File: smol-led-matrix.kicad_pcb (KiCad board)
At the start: 4 copper layers, 61.8 x 88.2 mm, 381 parts, among them J1 USB_C_Receptacle_USB2.0, J2 TagConnect_TC2030_SWD, Q1 FS8205, Q2 AO3401A, SW1 SW_Push, SW2 SW_Push, U1 STM32L433CBTx, U2 TP4054, U3 DW01+G, U4 XC6206P332MR

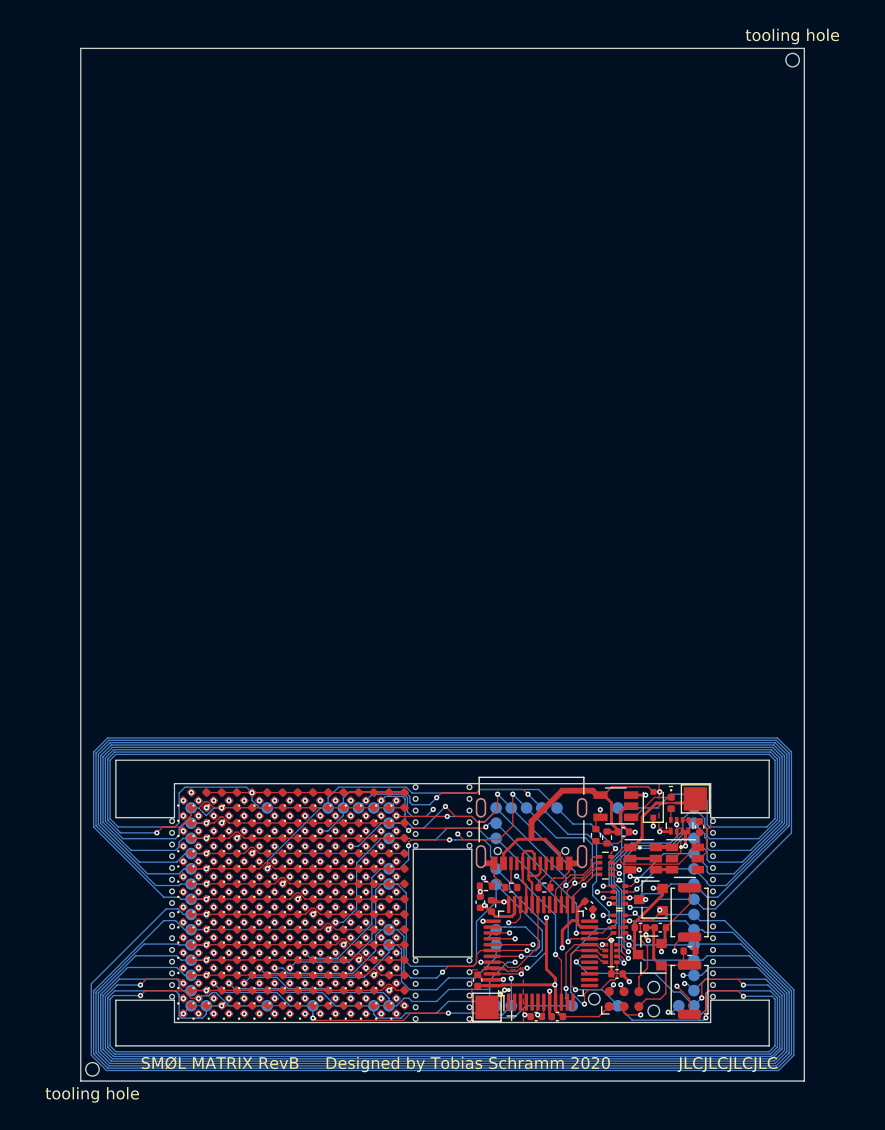
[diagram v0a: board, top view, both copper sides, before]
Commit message: Repanelize
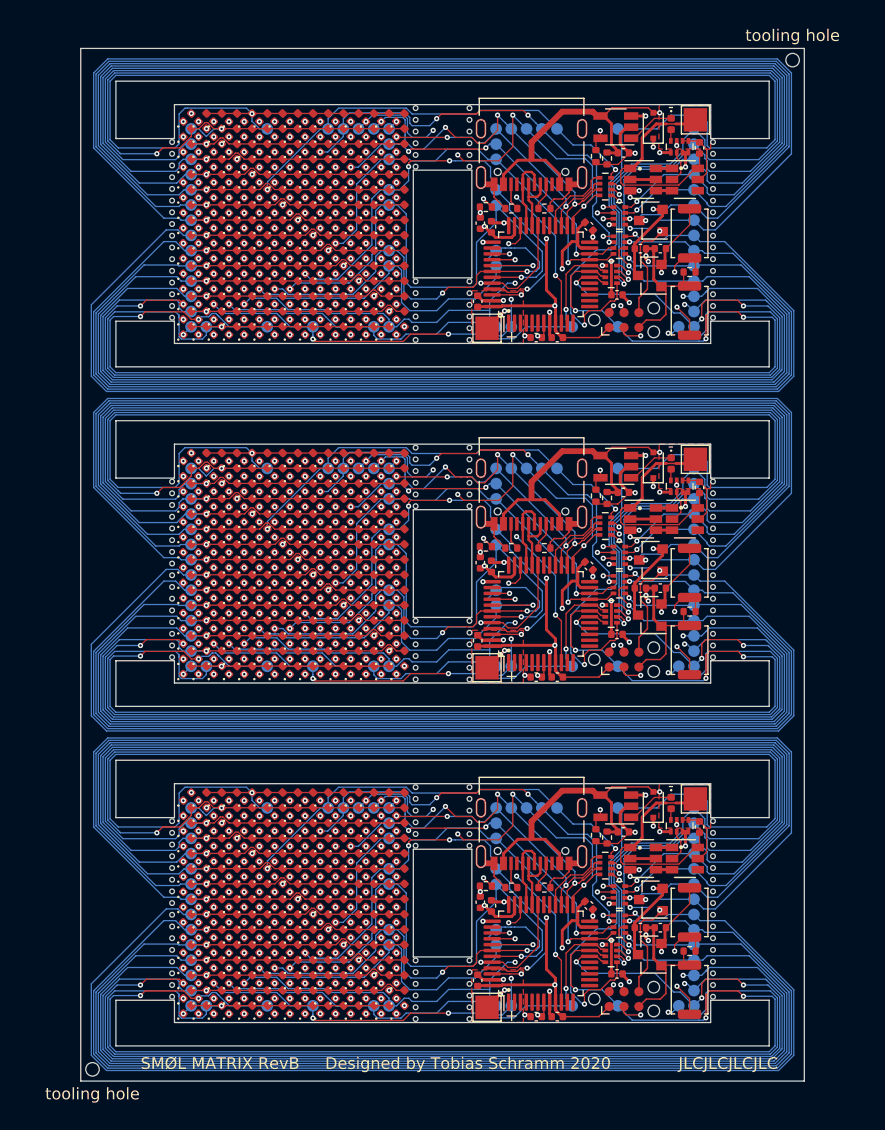
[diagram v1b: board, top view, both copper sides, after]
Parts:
- added C1: 100nF, Capacitor_SMD:C_0402_1005Metric, F.Cu at (94.8, 86.5)
- added C1: 100nF, Capacitor_SMD:C_0402_1005Metric, F.Cu at (94.8, 115.5)
- added C10: 10uF, Capacitor_SMD:C_0402_1005Metric, F.Cu at (99.9, 82.8)
- added C10: 10uF, Capacitor_SMD:C_0402_1005Metric, F.Cu at (99.9, 111.8)
- added C11: 100nF, Capacitor_SMD:C_0402_1005Metric, F.Cu at (88.2, 76.7)
- added C11: 100nF, Capacitor_SMD:C_0402_1005Metric, F.Cu at (88.2, 105.7)
- added C2: 100nF, Capacitor_SMD:C_0402_1005Metric, F.Cu at (88.0, 83.4)
- added C2: 100nF, Capacitor_SMD:C_0402_1005Metric, F.Cu at (88.0, 112.4)
- added C3: 1uF, Capacitor_SMD:C_0402_1005Metric, F.Cu at (100.5, 70.7)
- added C3: 1uF, Capacitor_SMD:C_0402_1005Metric, F.Cu at (100.5, 99.7)
- added C4: 100nF, Capacitor_SMD:C_0402_1005Metric, F.Cu at (107.0, 70.3)
- added C4: 100nF, Capacitor_SMD:C_0402_1005Metric, F.Cu at (107.0, 99.3)
- added C5: 100nF, Capacitor_SMD:C_0402_1005Metric, F.Cu at (93.0, 86.5)
- added C5: 100nF, Capacitor_SMD:C_0402_1005Metric, F.Cu at (93.0, 115.5)
- added C6: 1uF, Capacitor_SMD:C_0402_1005Metric, F.Cu at (101.9, 78.9)
- added C6: 1uF, Capacitor_SMD:C_0402_1005Metric, F.Cu at (101.9, 107.9)
- added C7: 1uF, Capacitor_SMD:C_0402_1005Metric, F.Cu at (103.6, 78.9)
- added C7: 1uF, Capacitor_SMD:C_0402_1005Metric, F.Cu at (103.6, 107.9)
- added C8: 100nF, Capacitor_SMD:C_0402_1005Metric, F.Cu at (89.2, 77.0)
- added C8: 100nF, Capacitor_SMD:C_0402_1005Metric, F.Cu at (89.2, 106.0)
- added C9: 100nF, Capacitor_SMD:C_0402_1005Metric, F.Cu at (97.5, 77.0)
- added C9: 100nF, Capacitor_SMD:C_0402_1005Metric, F.Cu at (97.5, 106.0)
- added D1: LED, LED_SMD:LED_0402_1005Metric, F.Cu at (63.2, 67.7)
- added D1: LED, LED_SMD:LED_0402_1005Metric, F.Cu at (63.2, 96.7)
- added D10: LED, LED_SMD:LED_0402_1005Metric, F.Cu at (63.2, 79.4)
- added D10: LED, LED_SMD:LED_0402_1005Metric, F.Cu at (63.2, 108.4)
- added D100: LED, LED_SMD:LED_0402_1005Metric, F.Cu at (71.0, 79.4)
- added D100: LED, LED_SMD:LED_0402_1005Metric, F.Cu at (71.0, 108.4)
- added D101: LED, LED_SMD:LED_0402_1005Metric, F.Cu at (71.0, 80.7)
- added D101: LED, LED_SMD:LED_0402_1005Metric, F.Cu at (71.0, 109.7)
- added D102: LED, LED_SMD:LED_0402_1005Metric, F.Cu at (71.0, 82.0)
- added D102: LED, LED_SMD:LED_0402_1005Metric, F.Cu at (71.0, 111.0)
- added D103: LED, LED_SMD:LED_0402_1005Metric, F.Cu at (71.0, 83.3)
- added D103: LED, LED_SMD:LED_0402_1005Metric, F.Cu at (71.0, 112.3)
- added D104: LED, LED_SMD:LED_0402_1005Metric, F.Cu at (71.0, 84.6)
- added D104: LED, LED_SMD:LED_0402_1005Metric, F.Cu at (71.0, 113.6)
- added D105: LED, LED_SMD:LED_0402_1005Metric, F.Cu at (71.0, 85.9)
- added D105: LED, LED_SMD:LED_0402_1005Metric, F.Cu at (71.0, 114.9)
- added D106: LED, LED_SMD:LED_0402_1005Metric, F.Cu at (72.3, 67.7)
- added D106: LED, LED_SMD:LED_0402_1005Metric, F.Cu at (72.3, 96.7)
- added D107: LED, LED_SMD:LED_0402_1005Metric, F.Cu at (72.3, 69.0)
- added D107: LED, LED_SMD:LED_0402_1005Metric, F.Cu at (72.3, 98.0)
- added D108: LED, LED_SMD:LED_0402_1005Metric, F.Cu at (72.3, 70.3)
- added D108: LED, LED_SMD:LED_0402_1005Metric, F.Cu at (72.3, 99.3)
- added D109: LED, LED_SMD:LED_0402_1005Metric, F.Cu at (72.3, 71.6)
- added D109: LED, LED_SMD:LED_0402_1005Metric, F.Cu at (72.3, 100.6)
- added D11: LED, LED_SMD:LED_0402_1005Metric, F.Cu at (63.2, 80.7)
- added D11: LED, LED_SMD:LED_0402_1005Metric, F.Cu at (63.2, 109.7)
- added D110: LED, LED_SMD:LED_0402_1005Metric, F.Cu at (72.3, 72.9)
- added D110: LED, LED_SMD:LED_0402_1005Metric, F.Cu at (72.3, 101.9)
- added D111: LED, LED_SMD:LED_0402_1005Metric, F.Cu at (72.3, 74.2)
- added D111: LED, LED_SMD:LED_0402_1005Metric, F.Cu at (72.3, 103.2)
- added D112: LED, LED_SMD:LED_0402_1005Metric, F.Cu at (72.3, 75.5)
- added D112: LED, LED_SMD:LED_0402_1005Metric, F.Cu at (72.3, 104.5)
- added D113: LED, LED_SMD:LED_0402_1005Metric, F.Cu at (72.3, 76.8)
- added D113: LED, LED_SMD:LED_0402_1005Metric, F.Cu at (72.3, 105.8)
- added D114: LED, LED_SMD:LED_0402_1005Metric, F.Cu at (72.3, 78.1)
- added D114: LED, LED_SMD:LED_0402_1005Metric, F.Cu at (72.3, 107.1)
- added D115: LED, LED_SMD:LED_0402_1005Metric, F.Cu at (72.3, 79.4)
- added D115: LED, LED_SMD:LED_0402_1005Metric, F.Cu at (72.3, 108.4)
- added D116: LED, LED_SMD:LED_0402_1005Metric, F.Cu at (72.3, 80.7)
- added D116: LED, LED_SMD:LED_0402_1005Metric, F.Cu at (72.3, 109.7)
- added D117: LED, LED_SMD:LED_0402_1005Metric, F.Cu at (72.3, 82.0)
- added D117: LED, LED_SMD:LED_0402_1005Metric, F.Cu at (72.3, 111.0)
- added D118: LED, LED_SMD:LED_0402_1005Metric, F.Cu at (72.3, 83.3)
- added D118: LED, LED_SMD:LED_0402_1005Metric, F.Cu at (72.3, 112.3)
- added D119: LED, LED_SMD:LED_0402_1005Metric, F.Cu at (72.3, 84.6)
- added D119: LED, LED_SMD:LED_0402_1005Metric, F.Cu at (72.3, 113.6)
- added D12: LED, LED_SMD:LED_0402_1005Metric, F.Cu at (63.2, 82.0)
- added D12: LED, LED_SMD:LED_0402_1005Metric, F.Cu at (63.2, 111.0)
- added D120: LED, LED_SMD:LED_0402_1005Metric, F.Cu at (72.3, 85.9)
- added D120: LED, LED_SMD:LED_0402_1005Metric, F.Cu at (72.3, 114.9)
- added D121: LED, LED_SMD:LED_0402_1005Metric, F.Cu at (73.6, 67.7)
- added D121: LED, LED_SMD:LED_0402_1005Metric, F.Cu at (73.6, 96.7)
- added D122: LED, LED_SMD:LED_0402_1005Metric, F.Cu at (73.6, 69.0)
- added D122: LED, LED_SMD:LED_0402_1005Metric, F.Cu at (73.6, 98.0)
- added D123: LED, LED_SMD:LED_0402_1005Metric, F.Cu at (73.6, 70.3)
- added D123: LED, LED_SMD:LED_0402_1005Metric, F.Cu at (73.6, 99.3)
- added D124: LED, LED_SMD:LED_0402_1005Metric, F.Cu at (73.6, 71.6)
- added D124: LED, LED_SMD:LED_0402_1005Metric, F.Cu at (73.6, 100.6)
- added D125: LED, LED_SMD:LED_0402_1005Metric, F.Cu at (73.6, 72.9)
- added D125: LED, LED_SMD:LED_0402_1005Metric, F.Cu at (73.6, 101.9)
- added D126: LED, LED_SMD:LED_0402_1005Metric, F.Cu at (73.6, 74.2)
- added D126: LED, LED_SMD:LED_0402_1005Metric, F.Cu at (73.6, 103.2)
- added D127: LED, LED_SMD:LED_0402_1005Metric, F.Cu at (73.6, 75.5)
- added D127: LED, LED_SMD:LED_0402_1005Metric, F.Cu at (73.6, 104.5)
- added D128: LED, LED_SMD:LED_0402_1005Metric, F.Cu at (73.6, 76.8)
- added D128: LED, LED_SMD:LED_0402_1005Metric, F.Cu at (73.6, 105.8)
- added D129: LED, LED_SMD:LED_0402_1005Metric, F.Cu at (73.6, 78.1)
- added D129: LED, LED_SMD:LED_0402_1005Metric, F.Cu at (73.6, 107.1)
- added D13: LED, LED_SMD:LED_0402_1005Metric, F.Cu at (63.2, 83.3)
- added D13: LED, LED_SMD:LED_0402_1005Metric, F.Cu at (63.2, 112.3)
- added D130: LED, LED_SMD:LED_0402_1005Metric, F.Cu at (73.6, 79.4)
- added D130: LED, LED_SMD:LED_0402_1005Metric, F.Cu at (73.6, 108.4)
- added D131: LED, LED_SMD:LED_0402_1005Metric, F.Cu at (73.6, 80.7)
- added D131: LED, LED_SMD:LED_0402_1005Metric, F.Cu at (73.6, 109.7)
- added D132: LED, LED_SMD:LED_0402_1005Metric, F.Cu at (73.6, 82.0)
- added D132: LED, LED_SMD:LED_0402_1005Metric, F.Cu at (73.6, 111.0)
- added D133: LED, LED_SMD:LED_0402_1005Metric, F.Cu at (73.6, 83.3)
- added D133: LED, LED_SMD:LED_0402_1005Metric, F.Cu at (73.6, 112.3)
- added D134: LED, LED_SMD:LED_0402_1005Metric, F.Cu at (73.6, 84.6)
- added D134: LED, LED_SMD:LED_0402_1005Metric, F.Cu at (73.6, 113.6)
- added D135: LED, LED_SMD:LED_0402_1005Metric, F.Cu at (73.6, 85.9)
- added D135: LED, LED_SMD:LED_0402_1005Metric, F.Cu at (73.6, 114.9)
- added D136: LED, LED_SMD:LED_0402_1005Metric, F.Cu at (74.9, 67.7)
- added D136: LED, LED_SMD:LED_0402_1005Metric, F.Cu at (74.9, 96.7)
- added D137: LED, LED_SMD:LED_0402_1005Metric, F.Cu at (74.9, 69.0)
- added D137: LED, LED_SMD:LED_0402_1005Metric, F.Cu at (74.9, 98.0)
- added D138: LED, LED_SMD:LED_0402_1005Metric, F.Cu at (74.9, 70.3)
- added D138: LED, LED_SMD:LED_0402_1005Metric, F.Cu at (74.9, 99.3)
- added D139: LED, LED_SMD:LED_0402_1005Metric, F.Cu at (74.9, 71.6)
- added D139: LED, LED_SMD:LED_0402_1005Metric, F.Cu at (74.9, 100.6)
- added D14: LED, LED_SMD:LED_0402_1005Metric, F.Cu at (63.2, 84.6)
- added D14: LED, LED_SMD:LED_0402_1005Metric, F.Cu at (63.2, 113.6)
- added D140: LED, LED_SMD:LED_0402_1005Metric, F.Cu at (74.9, 72.9)
- added D140: LED, LED_SMD:LED_0402_1005Metric, F.Cu at (74.9, 101.9)
- added D141: LED, LED_SMD:LED_0402_1005Metric, F.Cu at (74.9, 74.2)
- added D141: LED, LED_SMD:LED_0402_1005Metric, F.Cu at (74.9, 103.2)
- added D142: LED, LED_SMD:LED_0402_1005Metric, F.Cu at (74.9, 75.5)
- added D142: LED, LED_SMD:LED_0402_1005Metric, F.Cu at (74.9, 104.5)
- added D143: LED, LED_SMD:LED_0402_1005Metric, F.Cu at (74.9, 76.8)
- added D143: LED, LED_SMD:LED_0402_1005Metric, F.Cu at (74.9, 105.8)
- added D144: LED, LED_SMD:LED_0402_1005Metric, F.Cu at (74.9, 78.1)
- added D144: LED, LED_SMD:LED_0402_1005Metric, F.Cu at (74.9, 107.1)
- added D145: LED, LED_SMD:LED_0402_1005Metric, F.Cu at (74.9, 79.4)
- added D145: LED, LED_SMD:LED_0402_1005Metric, F.Cu at (74.9, 108.4)
- added D146: LED, LED_SMD:LED_0402_1005Metric, F.Cu at (74.9, 80.7)
- added D146: LED, LED_SMD:LED_0402_1005Metric, F.Cu at (74.9, 109.7)
- added D147: LED, LED_SMD:LED_0402_1005Metric, F.Cu at (74.9, 82.0)
- added D147: LED, LED_SMD:LED_0402_1005Metric, F.Cu at (74.9, 111.0)
- added D148: LED, LED_SMD:LED_0402_1005Metric, F.Cu at (74.9, 83.3)
- added D148: LED, LED_SMD:LED_0402_1005Metric, F.Cu at (74.9, 112.3)
- added D149: LED, LED_SMD:LED_0402_1005Metric, F.Cu at (74.9, 84.6)
- added D149: LED, LED_SMD:LED_0402_1005Metric, F.Cu at (74.9, 113.6)
- added D15: LED, LED_SMD:LED_0402_1005Metric, F.Cu at (63.2, 85.9)
- added D15: LED, LED_SMD:LED_0402_1005Metric, F.Cu at (63.2, 114.9)
- added D150: LED, LED_SMD:LED_0402_1005Metric, F.Cu at (74.9, 85.9)
- added D150: LED, LED_SMD:LED_0402_1005Metric, F.Cu at (74.9, 114.9)
- added D151: LED, LED_SMD:LED_0402_1005Metric, F.Cu at (76.2, 67.7)
- added D151: LED, LED_SMD:LED_0402_1005Metric, F.Cu at (76.2, 96.7)
- added D152: LED, LED_SMD:LED_0402_1005Metric, F.Cu at (76.2, 69.0)
- added D152: LED, LED_SMD:LED_0402_1005Metric, F.Cu at (76.2, 98.0)
- added D153: LED, LED_SMD:LED_0402_1005Metric, F.Cu at (76.2, 70.3)
- added D153: LED, LED_SMD:LED_0402_1005Metric, F.Cu at (76.2, 99.3)
- added D154: LED, LED_SMD:LED_0402_1005Metric, F.Cu at (76.2, 71.6)
- added D154: LED, LED_SMD:LED_0402_1005Metric, F.Cu at (76.2, 100.6)
- added D155: LED, LED_SMD:LED_0402_1005Metric, F.Cu at (76.2, 72.9)
- added D155: LED, LED_SMD:LED_0402_1005Metric, F.Cu at (76.2, 101.9)
- added D156: LED, LED_SMD:LED_0402_1005Metric, F.Cu at (76.2, 74.2)
- added D156: LED, LED_SMD:LED_0402_1005Metric, F.Cu at (76.2, 103.2)
- added D157: LED, LED_SMD:LED_0402_1005Metric, F.Cu at (76.2, 75.5)
- added D157: LED, LED_SMD:LED_0402_1005Metric, F.Cu at (76.2, 104.5)
- added D158: LED, LED_SMD:LED_0402_1005Metric, F.Cu at (76.2, 76.8)
- added D158: LED, LED_SMD:LED_0402_1005Metric, F.Cu at (76.2, 105.8)
- added D159: LED, LED_SMD:LED_0402_1005Metric, F.Cu at (76.2, 78.1)
- added D159: LED, LED_SMD:LED_0402_1005Metric, F.Cu at (76.2, 107.1)
- added D16: LED, LED_SMD:LED_0402_1005Metric, F.Cu at (64.5, 67.7)
- added D16: LED, LED_SMD:LED_0402_1005Metric, F.Cu at (64.5, 96.7)
- added D160: LED, LED_SMD:LED_0402_1005Metric, F.Cu at (76.2, 79.4)
- added D160: LED, LED_SMD:LED_0402_1005Metric, F.Cu at (76.2, 108.4)
- added D161: LED, LED_SMD:LED_0402_1005Metric, F.Cu at (76.2, 80.7)
- added D161: LED, LED_SMD:LED_0402_1005Metric, F.Cu at (76.2, 109.7)
- added D162: LED, LED_SMD:LED_0402_1005Metric, F.Cu at (76.2, 82.0)
- added D162: LED, LED_SMD:LED_0402_1005Metric, F.Cu at (76.2, 111.0)
- added D163: LED, LED_SMD:LED_0402_1005Metric, F.Cu at (76.2, 83.3)
- added D163: LED, LED_SMD:LED_0402_1005Metric, F.Cu at (76.2, 112.3)
- added D164: LED, LED_SMD:LED_0402_1005Metric, F.Cu at (76.2, 84.6)
- added D164: LED, LED_SMD:LED_0402_1005Metric, F.Cu at (76.2, 113.6)
- added D165: LED, LED_SMD:LED_0402_1005Metric, F.Cu at (76.2, 85.9)
- added D165: LED, LED_SMD:LED_0402_1005Metric, F.Cu at (76.2, 114.9)
- added D166: LED, LED_SMD:LED_0402_1005Metric, F.Cu at (77.5, 67.7)
- added D166: LED, LED_SMD:LED_0402_1005Metric, F.Cu at (77.5, 96.7)
- added D167: LED, LED_SMD:LED_0402_1005Metric, F.Cu at (77.5, 69.0)
- added D167: LED, LED_SMD:LED_0402_1005Metric, F.Cu at (77.5, 98.0)
- added D168: LED, LED_SMD:LED_0402_1005Metric, F.Cu at (77.5, 70.3)
- added D168: LED, LED_SMD:LED_0402_1005Metric, F.Cu at (77.5, 99.3)
- added D169: LED, LED_SMD:LED_0402_1005Metric, F.Cu at (77.5, 71.6)
- added D169: LED, LED_SMD:LED_0402_1005Metric, F.Cu at (77.5, 100.6)
- added D17: LED, LED_SMD:LED_0402_1005Metric, F.Cu at (64.5, 69.0)
- added D17: LED, LED_SMD:LED_0402_1005Metric, F.Cu at (64.5, 98.0)
- added D170: LED, LED_SMD:LED_0402_1005Metric, F.Cu at (77.5, 72.9)
- added D170: LED, LED_SMD:LED_0402_1005Metric, F.Cu at (77.5, 101.9)
- added D171: LED, LED_SMD:LED_0402_1005Metric, F.Cu at (77.5, 74.2)
- added D171: LED, LED_SMD:LED_0402_1005Metric, F.Cu at (77.5, 103.2)
- added D172: LED, LED_SMD:LED_0402_1005Metric, F.Cu at (77.5, 75.5)
- added D172: LED, LED_SMD:LED_0402_1005Metric, F.Cu at (77.5, 104.5)
- added D173: LED, LED_SMD:LED_0402_1005Metric, F.Cu at (77.5, 76.8)
- added D173: LED, LED_SMD:LED_0402_1005Metric, F.Cu at (77.5, 105.8)
- added D174: LED, LED_SMD:LED_0402_1005Metric, F.Cu at (77.5, 78.1)
- added D174: LED, LED_SMD:LED_0402_1005Metric, F.Cu at (77.5, 107.1)
- added D175: LED, LED_SMD:LED_0402_1005Metric, F.Cu at (77.5, 79.4)
- added D175: LED, LED_SMD:LED_0402_1005Metric, F.Cu at (77.5, 108.4)
- added D176: LED, LED_SMD:LED_0402_1005Metric, F.Cu at (77.5, 80.7)
- added D176: LED, LED_SMD:LED_0402_1005Metric, F.Cu at (77.5, 109.7)
- added D177: LED, LED_SMD:LED_0402_1005Metric, F.Cu at (77.5, 82.0)
- added D177: LED, LED_SMD:LED_0402_1005Metric, F.Cu at (77.5, 111.0)
- added D178: LED, LED_SMD:LED_0402_1005Metric, F.Cu at (77.5, 83.3)
- added D178: LED, LED_SMD:LED_0402_1005Metric, F.Cu at (77.5, 112.3)
- added D179: LED, LED_SMD:LED_0402_1005Metric, F.Cu at (77.5, 84.6)
- added D179: LED, LED_SMD:LED_0402_1005Metric, F.Cu at (77.5, 113.6)
- added D18: LED, LED_SMD:LED_0402_1005Metric, F.Cu at (64.5, 70.3)
- added D18: LED, LED_SMD:LED_0402_1005Metric, F.Cu at (64.5, 99.3)
- added D180: LED, LED_SMD:LED_0402_1005Metric, F.Cu at (77.5, 85.9)
- added D180: LED, LED_SMD:LED_0402_1005Metric, F.Cu at (77.5, 114.9)
- added D181: LED, LED_SMD:LED_0402_1005Metric, F.Cu at (78.8, 67.7)
- added D181: LED, LED_SMD:LED_0402_1005Metric, F.Cu at (78.8, 96.7)
- added D182: LED, LED_SMD:LED_0402_1005Metric, F.Cu at (78.8, 69.0)
- added D182: LED, LED_SMD:LED_0402_1005Metric, F.Cu at (78.8, 98.0)
- added D183: LED, LED_SMD:LED_0402_1005Metric, F.Cu at (78.8, 70.3)
- added D183: LED, LED_SMD:LED_0402_1005Metric, F.Cu at (78.8, 99.3)
- added D184: LED, LED_SMD:LED_0402_1005Metric, F.Cu at (78.8, 71.6)
- added D184: LED, LED_SMD:LED_0402_1005Metric, F.Cu at (78.8, 100.6)
- added D185: LED, LED_SMD:LED_0402_1005Metric, F.Cu at (78.8, 72.9)
- added D185: LED, LED_SMD:LED_0402_1005Metric, F.Cu at (78.8, 101.9)
- added D186: LED, LED_SMD:LED_0402_1005Metric, F.Cu at (78.8, 74.2)
- added D186: LED, LED_SMD:LED_0402_1005Metric, F.Cu at (78.8, 103.2)
- added D187: LED, LED_SMD:LED_0402_1005Metric, F.Cu at (78.8, 75.5)
- added D187: LED, LED_SMD:LED_0402_1005Metric, F.Cu at (78.8, 104.5)
- added D188: LED, LED_SMD:LED_0402_1005Metric, F.Cu at (78.8, 76.8)
- added D188: LED, LED_SMD:LED_0402_1005Metric, F.Cu at (78.8, 105.8)
- added D189: LED, LED_SMD:LED_0402_1005Metric, F.Cu at (78.8, 78.1)
- added D189: LED, LED_SMD:LED_0402_1005Metric, F.Cu at (78.8, 107.1)
- added D19: LED, LED_SMD:LED_0402_1005Metric, F.Cu at (64.5, 71.6)
- added D19: LED, LED_SMD:LED_0402_1005Metric, F.Cu at (64.5, 100.6)
- added D190: LED, LED_SMD:LED_0402_1005Metric, F.Cu at (78.8, 79.4)
- added D190: LED, LED_SMD:LED_0402_1005Metric, F.Cu at (78.8, 108.4)
- added D191: LED, LED_SMD:LED_0402_1005Metric, F.Cu at (78.8, 80.7)
- added D191: LED, LED_SMD:LED_0402_1005Metric, F.Cu at (78.8, 109.7)
- added D192: LED, LED_SMD:LED_0402_1005Metric, F.Cu at (78.8, 82.0)
- added D192: LED, LED_SMD:LED_0402_1005Metric, F.Cu at (78.8, 111.0)
- added D193: LED, LED_SMD:LED_0402_1005Metric, F.Cu at (78.8, 83.3)
- added D193: LED, LED_SMD:LED_0402_1005Metric, F.Cu at (78.8, 112.3)
- added D194: LED, LED_SMD:LED_0402_1005Metric, F.Cu at (78.8, 84.6)
- added D194: LED, LED_SMD:LED_0402_1005Metric, F.Cu at (78.8, 113.6)
- added D195: LED, LED_SMD:LED_0402_1005Metric, F.Cu at (78.8, 85.9)
- added D195: LED, LED_SMD:LED_0402_1005Metric, F.Cu at (78.8, 114.9)
- added D196: LED, LED_SMD:LED_0402_1005Metric, F.Cu at (80.1, 67.7)
- added D196: LED, LED_SMD:LED_0402_1005Metric, F.Cu at (80.1, 96.7)
- added D197: LED, LED_SMD:LED_0402_1005Metric, F.Cu at (80.1, 69.0)
- added D197: LED, LED_SMD:LED_0402_1005Metric, F.Cu at (80.1, 98.0)
- added D198: LED, LED_SMD:LED_0402_1005Metric, F.Cu at (80.1, 70.3)
- added D198: LED, LED_SMD:LED_0402_1005Metric, F.Cu at (80.1, 99.3)
- added D199: LED, LED_SMD:LED_0402_1005Metric, F.Cu at (80.1, 71.6)
- added D199: LED, LED_SMD:LED_0402_1005Metric, F.Cu at (80.1, 100.6)
- added D2: LED, LED_SMD:LED_0402_1005Metric, F.Cu at (63.2, 69.0)
- added D2: LED, LED_SMD:LED_0402_1005Metric, F.Cu at (63.2, 98.0)
- added D20: LED, LED_SMD:LED_0402_1005Metric, F.Cu at (64.5, 72.9)
- added D20: LED, LED_SMD:LED_0402_1005Metric, F.Cu at (64.5, 101.9)
- added D200: LED, LED_SMD:LED_0402_1005Metric, F.Cu at (80.1, 72.9)
- added D200: LED, LED_SMD:LED_0402_1005Metric, F.Cu at (80.1, 101.9)
- added D201: LED, LED_SMD:LED_0402_1005Metric, F.Cu at (80.1, 74.2)
- added D201: LED, LED_SMD:LED_0402_1005Metric, F.Cu at (80.1, 103.2)
- added D202: LED, LED_SMD:LED_0402_1005Metric, F.Cu at (80.1, 75.5)
- added D202: LED, LED_SMD:LED_0402_1005Metric, F.Cu at (80.1, 104.5)
- added D203: LED, LED_SMD:LED_0402_1005Metric, F.Cu at (80.1, 76.8)
- added D203: LED, LED_SMD:LED_0402_1005Metric, F.Cu at (80.1, 105.8)
- added D204: LED, LED_SMD:LED_0402_1005Metric, F.Cu at (80.1, 78.1)
- added D204: LED, LED_SMD:LED_0402_1005Metric, F.Cu at (80.1, 107.1)
- added D205: LED, LED_SMD:LED_0402_1005Metric, F.Cu at (80.1, 79.4)
- added D205: LED, LED_SMD:LED_0402_1005Metric, F.Cu at (80.1, 108.4)
- added D206: LED, LED_SMD:LED_0402_1005Metric, F.Cu at (80.1, 80.7)
- added D206: LED, LED_SMD:LED_0402_1005Metric, F.Cu at (80.1, 109.7)
- added D207: LED, LED_SMD:LED_0402_1005Metric, F.Cu at (80.1, 82.0)
- added D207: LED, LED_SMD:LED_0402_1005Metric, F.Cu at (80.1, 111.0)
- added D208: LED, LED_SMD:LED_0402_1005Metric, F.Cu at (80.1, 83.3)
- added D208: LED, LED_SMD:LED_0402_1005Metric, F.Cu at (80.1, 112.3)
- added D209: LED, LED_SMD:LED_0402_1005Metric, F.Cu at (80.1, 84.6)
- added D209: LED, LED_SMD:LED_0402_1005Metric, F.Cu at (80.1, 113.6)
- added D21: LED, LED_SMD:LED_0402_1005Metric, F.Cu at (64.5, 74.2)
- added D21: LED, LED_SMD:LED_0402_1005Metric, F.Cu at (64.5, 103.2)
- added D210: LED, LED_SMD:LED_0402_1005Metric, F.Cu at (80.1, 85.9)
- added D210: LED, LED_SMD:LED_0402_1005Metric, F.Cu at (80.1, 114.9)
- added D211: LED, LED_SMD:LED_0402_1005Metric, F.Cu at (81.4, 67.7)
- added D211: LED, LED_SMD:LED_0402_1005Metric, F.Cu at (81.4, 96.7)
- added D212: LED, LED_SMD:LED_0402_1005Metric, F.Cu at (81.4, 69.0)
- added D212: LED, LED_SMD:LED_0402_1005Metric, F.Cu at (81.4, 98.0)
- added D213: LED, LED_SMD:LED_0402_1005Metric, F.Cu at (81.4, 70.3)
- added D213: LED, LED_SMD:LED_0402_1005Metric, F.Cu at (81.4, 99.3)
- added D214: LED, LED_SMD:LED_0402_1005Metric, F.Cu at (81.4, 71.6)
- added D214: LED, LED_SMD:LED_0402_1005Metric, F.Cu at (81.4, 100.6)
- added D215: LED, LED_SMD:LED_0402_1005Metric, F.Cu at (81.4, 72.9)
- added D215: LED, LED_SMD:LED_0402_1005Metric, F.Cu at (81.4, 101.9)
- added D216: LED, LED_SMD:LED_0402_1005Metric, F.Cu at (81.4, 74.2)
- added D216: LED, LED_SMD:LED_0402_1005Metric, F.Cu at (81.4, 103.2)
- added D217: LED, LED_SMD:LED_0402_1005Metric, F.Cu at (81.4, 75.5)
- added D217: LED, LED_SMD:LED_0402_1005Metric, F.Cu at (81.4, 104.5)
- added D218: LED, LED_SMD:LED_0402_1005Metric, F.Cu at (81.4, 76.8)
- added D218: LED, LED_SMD:LED_0402_1005Metric, F.Cu at (81.4, 105.8)
- added D219: LED, LED_SMD:LED_0402_1005Metric, F.Cu at (81.4, 78.1)
- added D219: LED, LED_SMD:LED_0402_1005Metric, F.Cu at (81.4, 107.1)
- added D22: LED, LED_SMD:LED_0402_1005Metric, F.Cu at (64.5, 75.5)
- added D22: LED, LED_SMD:LED_0402_1005Metric, F.Cu at (64.5, 104.5)
- added D220: LED, LED_SMD:LED_0402_1005Metric, F.Cu at (81.4, 79.4)
- added D220: LED, LED_SMD:LED_0402_1005Metric, F.Cu at (81.4, 108.4)
- added D221: LED, LED_SMD:LED_0402_1005Metric, F.Cu at (81.4, 80.7)
- added D221: LED, LED_SMD:LED_0402_1005Metric, F.Cu at (81.4, 109.7)
- added D222: LED, LED_SMD:LED_0402_1005Metric, F.Cu at (81.4, 82.0)
- added D222: LED, LED_SMD:LED_0402_1005Metric, F.Cu at (81.4, 111.0)
- added D223: LED, LED_SMD:LED_0402_1005Metric, F.Cu at (81.4, 83.3)
- added D223: LED, LED_SMD:LED_0402_1005Metric, F.Cu at (81.4, 112.3)
- added D224: LED, LED_SMD:LED_0402_1005Metric, F.Cu at (81.4, 84.6)
- added D224: LED, LED_SMD:LED_0402_1005Metric, F.Cu at (81.4, 113.6)
- added D225: LED, LED_SMD:LED_0402_1005Metric, F.Cu at (81.4, 85.9)
- added D225: LED, LED_SMD:LED_0402_1005Metric, F.Cu at (81.4, 114.9)
- added D226: LED, LED_SMD:LED_0402_1005Metric, F.Cu at (104.5, 68.2)
- added D226: LED, LED_SMD:LED_0402_1005Metric, F.Cu at (104.5, 97.2)
- added D227: 1N4148, Diode_SMD:D_SOD-323F, F.Cu at (103.0, 68.4)
- added D227: 1N4148, Diode_SMD:D_SOD-323F, F.Cu at (103.0, 97.4)
- added D23: LED, LED_SMD:LED_0402_1005Metric, F.Cu at (64.5, 76.8)
- added D23: LED, LED_SMD:LED_0402_1005Metric, F.Cu at (64.5, 105.8)
- added D24: LED, LED_SMD:LED_0402_1005Metric, F.Cu at (64.5, 78.1)
- added D24: LED, LED_SMD:LED_0402_1005Metric, F.Cu at (64.5, 107.1)
- added D25: LED, LED_SMD:LED_0402_1005Metric, F.Cu at (64.5, 79.4)
- added D25: LED, LED_SMD:LED_0402_1005Metric, F.Cu at (64.5, 108.4)
- added D26: LED, LED_SMD:LED_0402_1005Metric, F.Cu at (64.5, 80.7)
- added D26: LED, LED_SMD:LED_0402_1005Metric, F.Cu at (64.5, 109.7)
- added D27: LED, LED_SMD:LED_0402_1005Metric, F.Cu at (64.5, 82.0)
- added D27: LED, LED_SMD:LED_0402_1005Metric, F.Cu at (64.5, 111.0)
- added D28: LED, LED_SMD:LED_0402_1005Metric, F.Cu at (64.5, 83.3)
- added D28: LED, LED_SMD:LED_0402_1005Metric, F.Cu at (64.5, 112.3)
- added D29: LED, LED_SMD:LED_0402_1005Metric, F.Cu at (64.5, 84.6)
- added D29: LED, LED_SMD:LED_0402_1005Metric, F.Cu at (64.5, 113.6)
- added D3: LED, LED_SMD:LED_0402_1005Metric, F.Cu at (63.2, 70.3)
- added D3: LED, LED_SMD:LED_0402_1005Metric, F.Cu at (63.2, 99.3)
- added D30: LED, LED_SMD:LED_0402_1005Metric, F.Cu at (64.5, 85.9)
- added D30: LED, LED_SMD:LED_0402_1005Metric, F.Cu at (64.5, 114.9)
- added D31: LED, LED_SMD:LED_0402_1005Metric, F.Cu at (65.8, 67.7)
- added D31: LED, LED_SMD:LED_0402_1005Metric, F.Cu at (65.8, 96.7)
- added D32: LED, LED_SMD:LED_0402_1005Metric, F.Cu at (65.8, 69.0)
- added D32: LED, LED_SMD:LED_0402_1005Metric, F.Cu at (65.8, 98.0)
- added D33: LED, LED_SMD:LED_0402_1005Metric, F.Cu at (65.8, 70.3)
- added D33: LED, LED_SMD:LED_0402_1005Metric, F.Cu at (65.8, 99.3)
- added D34: LED, LED_SMD:LED_0402_1005Metric, F.Cu at (65.8, 71.6)
- added D34: LED, LED_SMD:LED_0402_1005Metric, F.Cu at (65.8, 100.6)
- added D35: LED, LED_SMD:LED_0402_1005Metric, F.Cu at (65.8, 72.9)
- added D35: LED, LED_SMD:LED_0402_1005Metric, F.Cu at (65.8, 101.9)
- added D36: LED, LED_SMD:LED_0402_1005Metric, F.Cu at (65.8, 74.2)
- added D36: LED, LED_SMD:LED_0402_1005Metric, F.Cu at (65.8, 103.2)
- added D37: LED, LED_SMD:LED_0402_1005Metric, F.Cu at (65.8, 75.5)
- added D37: LED, LED_SMD:LED_0402_1005Metric, F.Cu at (65.8, 104.5)
- added D38: LED, LED_SMD:LED_0402_1005Metric, F.Cu at (65.8, 76.8)
- added D38: LED, LED_SMD:LED_0402_1005Metric, F.Cu at (65.8, 105.8)
- added D39: LED, LED_SMD:LED_0402_1005Metric, F.Cu at (65.8, 78.1)
- added D39: LED, LED_SMD:LED_0402_1005Metric, F.Cu at (65.8, 107.1)
- added D4: LED, LED_SMD:LED_0402_1005Metric, F.Cu at (63.2, 71.6)
- added D4: LED, LED_SMD:LED_0402_1005Metric, F.Cu at (63.2, 100.6)
- added D40: LED, LED_SMD:LED_0402_1005Metric, F.Cu at (65.8, 79.4)
- added D40: LED, LED_SMD:LED_0402_1005Metric, F.Cu at (65.8, 108.4)
- added D41: LED, LED_SMD:LED_0402_1005Metric, F.Cu at (65.8, 80.7)
- added D41: LED, LED_SMD:LED_0402_1005Metric, F.Cu at (65.8, 109.7)
- added D42: LED, LED_SMD:LED_0402_1005Metric, F.Cu at (65.8, 82.0)
- added D42: LED, LED_SMD:LED_0402_1005Metric, F.Cu at (65.8, 111.0)
- added D43: LED, LED_SMD:LED_0402_1005Metric, F.Cu at (65.8, 83.3)
- added D43: LED, LED_SMD:LED_0402_1005Metric, F.Cu at (65.8, 112.3)
- added D44: LED, LED_SMD:LED_0402_1005Metric, F.Cu at (65.8, 84.6)
- added D44: LED, LED_SMD:LED_0402_1005Metric, F.Cu at (65.8, 113.6)
- added D45: LED, LED_SMD:LED_0402_1005Metric, F.Cu at (65.8, 85.9)
- added D45: LED, LED_SMD:LED_0402_1005Metric, F.Cu at (65.8, 114.9)
- added D46: LED, LED_SMD:LED_0402_1005Metric, F.Cu at (67.1, 67.7)
- added D46: LED, LED_SMD:LED_0402_1005Metric, F.Cu at (67.1, 96.7)
- added D47: LED, LED_SMD:LED_0402_1005Metric, F.Cu at (67.1, 69.0)
- added D47: LED, LED_SMD:LED_0402_1005Metric, F.Cu at (67.1, 98.0)
- added D48: LED, LED_SMD:LED_0402_1005Metric, F.Cu at (67.1, 70.3)
- added D48: LED, LED_SMD:LED_0402_1005Metric, F.Cu at (67.1, 99.3)
- added D49: LED, LED_SMD:LED_0402_1005Metric, F.Cu at (67.1, 71.6)
- added D49: LED, LED_SMD:LED_0402_1005Metric, F.Cu at (67.1, 100.6)
- added D5: LED, LED_SMD:LED_0402_1005Metric, F.Cu at (63.2, 72.9)
- added D5: LED, LED_SMD:LED_0402_1005Metric, F.Cu at (63.2, 101.9)
- added D50: LED, LED_SMD:LED_0402_1005Metric, F.Cu at (67.1, 72.9)
- added D50: LED, LED_SMD:LED_0402_1005Metric, F.Cu at (67.1, 101.9)
- added D51: LED, LED_SMD:LED_0402_1005Metric, F.Cu at (67.1, 74.2)
- added D51: LED, LED_SMD:LED_0402_1005Metric, F.Cu at (67.1, 103.2)
- added D52: LED, LED_SMD:LED_0402_1005Metric, F.Cu at (67.1, 75.5)
- added D52: LED, LED_SMD:LED_0402_1005Metric, F.Cu at (67.1, 104.5)
- added D53: LED, LED_SMD:LED_0402_1005Metric, F.Cu at (67.1, 76.8)
- added D53: LED, LED_SMD:LED_0402_1005Metric, F.Cu at (67.1, 105.8)
- added D54: LED, LED_SMD:LED_0402_1005Metric, F.Cu at (67.1, 78.1)
- added D54: LED, LED_SMD:LED_0402_1005Metric, F.Cu at (67.1, 107.1)
- added D55: LED, LED_SMD:LED_0402_1005Metric, F.Cu at (67.1, 79.4)
- added D55: LED, LED_SMD:LED_0402_1005Metric, F.Cu at (67.1, 108.4)
- added D56: LED, LED_SMD:LED_0402_1005Metric, F.Cu at (67.1, 80.7)
- added D56: LED, LED_SMD:LED_0402_1005Metric, F.Cu at (67.1, 109.7)
- added D57: LED, LED_SMD:LED_0402_1005Metric, F.Cu at (67.1, 82.0)
- added D57: LED, LED_SMD:LED_0402_1005Metric, F.Cu at (67.1, 111.0)
- added D58: LED, LED_SMD:LED_0402_1005Metric, F.Cu at (67.1, 83.3)
- added D58: LED, LED_SMD:LED_0402_1005Metric, F.Cu at (67.1, 112.3)
- added D59: LED, LED_SMD:LED_0402_1005Metric, F.Cu at (67.1, 84.6)
- added D59: LED, LED_SMD:LED_0402_1005Metric, F.Cu at (67.1, 113.6)
- added D6: LED, LED_SMD:LED_0402_1005Metric, F.Cu at (63.2, 74.2)
- added D6: LED, LED_SMD:LED_0402_1005Metric, F.Cu at (63.2, 103.2)
- added D60: LED, LED_SMD:LED_0402_1005Metric, F.Cu at (67.1, 85.9)
- added D60: LED, LED_SMD:LED_0402_1005Metric, F.Cu at (67.1, 114.9)
- added D61: LED, LED_SMD:LED_0402_1005Metric, F.Cu at (68.4, 67.7)
- added D61: LED, LED_SMD:LED_0402_1005Metric, F.Cu at (68.4, 96.7)
- added D62: LED, LED_SMD:LED_0402_1005Metric, F.Cu at (68.4, 69.0)
- added D62: LED, LED_SMD:LED_0402_1005Metric, F.Cu at (68.4, 98.0)
- added D63: LED, LED_SMD:LED_0402_1005Metric, F.Cu at (68.4, 70.3)
- added D63: LED, LED_SMD:LED_0402_1005Metric, F.Cu at (68.4, 99.3)
- added D64: LED, LED_SMD:LED_0402_1005Metric, F.Cu at (68.4, 71.6)
- added D64: LED, LED_SMD:LED_0402_1005Metric, F.Cu at (68.4, 100.6)
- added D65: LED, LED_SMD:LED_0402_1005Metric, F.Cu at (68.4, 72.9)
- added D65: LED, LED_SMD:LED_0402_1005Metric, F.Cu at (68.4, 101.9)
- added D66: LED, LED_SMD:LED_0402_1005Metric, F.Cu at (68.4, 74.2)
- added D66: LED, LED_SMD:LED_0402_1005Metric, F.Cu at (68.4, 103.2)
- added D67: LED, LED_SMD:LED_0402_1005Metric, F.Cu at (68.4, 75.5)
- added D67: LED, LED_SMD:LED_0402_1005Metric, F.Cu at (68.4, 104.5)
- added D68: LED, LED_SMD:LED_0402_1005Metric, F.Cu at (68.4, 76.8)
- added D68: LED, LED_SMD:LED_0402_1005Metric, F.Cu at (68.4, 105.8)
- added D69: LED, LED_SMD:LED_0402_1005Metric, F.Cu at (68.4, 78.1)
- added D69: LED, LED_SMD:LED_0402_1005Metric, F.Cu at (68.4, 107.1)
- added D7: LED, LED_SMD:LED_0402_1005Metric, F.Cu at (63.2, 75.5)
- added D7: LED, LED_SMD:LED_0402_1005Metric, F.Cu at (63.2, 104.5)
- added D70: LED, LED_SMD:LED_0402_1005Metric, F.Cu at (68.4, 79.4)
- added D70: LED, LED_SMD:LED_0402_1005Metric, F.Cu at (68.4, 108.4)
- added D71: LED, LED_SMD:LED_0402_1005Metric, F.Cu at (68.4, 80.7)
- added D71: LED, LED_SMD:LED_0402_1005Metric, F.Cu at (68.4, 109.7)
- added D72: LED, LED_SMD:LED_0402_1005Metric, F.Cu at (68.4, 82.0)
- added D72: LED, LED_SMD:LED_0402_1005Metric, F.Cu at (68.4, 111.0)
- added D73: LED, LED_SMD:LED_0402_1005Metric, F.Cu at (68.4, 83.3)
- added D73: LED, LED_SMD:LED_0402_1005Metric, F.Cu at (68.4, 112.3)
- added D74: LED, LED_SMD:LED_0402_1005Metric, F.Cu at (68.4, 84.6)
- added D74: LED, LED_SMD:LED_0402_1005Metric, F.Cu at (68.4, 113.6)
- added D75: LED, LED_SMD:LED_0402_1005Metric, F.Cu at (68.4, 85.9)
- added D75: LED, LED_SMD:LED_0402_1005Metric, F.Cu at (68.4, 114.9)
- added D76: LED, LED_SMD:LED_0402_1005Metric, F.Cu at (69.7, 67.7)
- added D76: LED, LED_SMD:LED_0402_1005Metric, F.Cu at (69.7, 96.7)
- added D77: LED, LED_SMD:LED_0402_1005Metric, F.Cu at (69.7, 69.0)
- added D77: LED, LED_SMD:LED_0402_1005Metric, F.Cu at (69.7, 98.0)
- added D78: LED, LED_SMD:LED_0402_1005Metric, F.Cu at (69.7, 70.3)
- added D78: LED, LED_SMD:LED_0402_1005Metric, F.Cu at (69.7, 99.3)
- added D79: LED, LED_SMD:LED_0402_1005Metric, F.Cu at (69.7, 71.6)
- added D79: LED, LED_SMD:LED_0402_1005Metric, F.Cu at (69.7, 100.6)
- added D8: LED, LED_SMD:LED_0402_1005Metric, F.Cu at (63.2, 76.8)
- added D8: LED, LED_SMD:LED_0402_1005Metric, F.Cu at (63.2, 105.8)
- added D80: LED, LED_SMD:LED_0402_1005Metric, F.Cu at (69.7, 72.9)
- added D80: LED, LED_SMD:LED_0402_1005Metric, F.Cu at (69.7, 101.9)
- added D81: LED, LED_SMD:LED_0402_1005Metric, F.Cu at (69.7, 74.2)
- added D81: LED, LED_SMD:LED_0402_1005Metric, F.Cu at (69.7, 103.2)
- added D82: LED, LED_SMD:LED_0402_1005Metric, F.Cu at (69.7, 75.5)
- added D82: LED, LED_SMD:LED_0402_1005Metric, F.Cu at (69.7, 104.5)
- added D83: LED, LED_SMD:LED_0402_1005Metric, F.Cu at (69.7, 76.8)
- added D83: LED, LED_SMD:LED_0402_1005Metric, F.Cu at (69.7, 105.8)
- added D84: LED, LED_SMD:LED_0402_1005Metric, F.Cu at (69.7, 78.1)
- added D84: LED, LED_SMD:LED_0402_1005Metric, F.Cu at (69.7, 107.1)
- added D85: LED, LED_SMD:LED_0402_1005Metric, F.Cu at (69.7, 79.4)
- added D85: LED, LED_SMD:LED_0402_1005Metric, F.Cu at (69.7, 108.4)
- added D86: LED, LED_SMD:LED_0402_1005Metric, F.Cu at (69.7, 80.7)
- added D86: LED, LED_SMD:LED_0402_1005Metric, F.Cu at (69.7, 109.7)
- added D87: LED, LED_SMD:LED_0402_1005Metric, F.Cu at (69.7, 82.0)
- added D87: LED, LED_SMD:LED_0402_1005Metric, F.Cu at (69.7, 111.0)
- added D88: LED, LED_SMD:LED_0402_1005Metric, F.Cu at (69.7, 83.3)
- added D88: LED, LED_SMD:LED_0402_1005Metric, F.Cu at (69.7, 112.3)
- added D89: LED, LED_SMD:LED_0402_1005Metric, F.Cu at (69.7, 84.6)
- added D89: LED, LED_SMD:LED_0402_1005Metric, F.Cu at (69.7, 113.6)
- added D9: LED, LED_SMD:LED_0402_1005Metric, F.Cu at (63.2, 78.1)
- added D9: LED, LED_SMD:LED_0402_1005Metric, F.Cu at (63.2, 107.1)
- added D90: LED, LED_SMD:LED_0402_1005Metric, F.Cu at (69.7, 85.9)
- added D90: LED, LED_SMD:LED_0402_1005Metric, F.Cu at (69.7, 114.9)
- added D91: LED, LED_SMD:LED_0402_1005Metric, F.Cu at (71.0, 67.7)
- added D91: LED, LED_SMD:LED_0402_1005Metric, F.Cu at (71.0, 96.7)
- added D92: LED, LED_SMD:LED_0402_1005Metric, F.Cu at (71.0, 69.0)
- added D92: LED, LED_SMD:LED_0402_1005Metric, F.Cu at (71.0, 98.0)
- added D93: LED, LED_SMD:LED_0402_1005Metric, F.Cu at (71.0, 70.3)
- added D93: LED, LED_SMD:LED_0402_1005Metric, F.Cu at (71.0, 99.3)
- added D94: LED, LED_SMD:LED_0402_1005Metric, F.Cu at (71.0, 71.6)
- added D94: LED, LED_SMD:LED_0402_1005Metric, F.Cu at (71.0, 100.6)
- added D95: LED, LED_SMD:LED_0402_1005Metric, F.Cu at (71.0, 72.9)
- added D95: LED, LED_SMD:LED_0402_1005Metric, F.Cu at (71.0, 101.9)
- added D96: LED, LED_SMD:LED_0402_1005Metric, F.Cu at (71.0, 74.2)
- added D96: LED, LED_SMD:LED_0402_1005Metric, F.Cu at (71.0, 103.2)
- added D97: LED, LED_SMD:LED_0402_1005Metric, F.Cu at (71.0, 75.5)
- added D97: LED, LED_SMD:LED_0402_1005Metric, F.Cu at (71.0, 104.5)
- added D98: LED, LED_SMD:LED_0402_1005Metric, F.Cu at (71.0, 76.8)
- added D98: LED, LED_SMD:LED_0402_1005Metric, F.Cu at (71.0, 105.8)
- added D99: LED, LED_SMD:LED_0402_1005Metric, F.Cu at (71.0, 78.1)
- added D99: LED, LED_SMD:LED_0402_1005Metric, F.Cu at (71.0, 107.1)
- added J1: USB_C_Receptacle_USB2.0, Connector_USB:USB_C_Receptacle_Palconn_UTC16-G, F.Cu at (92.6, 70.9)
- added J1: USB_C_Receptacle_USB2.0, Connector_USB:USB_C_Receptacle_Palconn_UTC16-G, F.Cu at (92.6, 99.9)
- added J2: TagConnect_TC2030_SWD, Connector:Tag-Connect_TC2030-IDC-NL_2x03_P1.27mm_Vertical, F.Cu at (100.5, 85.0)
- added J2: TagConnect_TC2030_SWD, Connector:Tag-Connect_TC2030-IDC-NL_2x03_P1.27mm_Vertical, F.Cu at (100.5, 114.0)
- added Q1: FS8205, Package_TO_SOT_SMD:SOT-23-6, F.Cu at (102.1, 73.0)
- added Q1: FS8205, Package_TO_SOT_SMD:SOT-23-6, F.Cu at (102.1, 102.0)
- added Q2: AO3401A, Package_TO_SOT_SMD:SOT-23, F.Cu at (102.8, 76.5)
- added Q2: AO3401A, Package_TO_SOT_SMD:SOT-23, F.Cu at (102.8, 105.5)
- added R1: 22kR, Resistor_SMD:R_0402_1005Metric, F.Cu at (98.1, 71.0)
- added R1: 22kR, Resistor_SMD:R_0402_1005Metric, F.Cu at (98.1, 100.0)
- added R2: 22kR, Resistor_SMD:R_0402_1005Metric, F.Cu at (99.0, 71.2)
- added R2: 22kR, Resistor_SMD:R_0402_1005Metric, F.Cu at (99.0, 100.2)
- added R3: 5.1kR, Resistor_SMD:R_0402_1005Metric, F.Cu at (93.7, 75.5)
- added R3: 5.1kR, Resistor_SMD:R_0402_1005Metric, F.Cu at (93.7, 104.5)
- added R4: 5.1kR, Resistor_SMD:R_0402_1005Metric, F.Cu at (90.9, 75.5)
- added R4: 5.1kR, Resistor_SMD:R_0402_1005Metric, F.Cu at (90.9, 104.5)
- added R5: 22kR, Resistor_SMD:R_0402_1005Metric, F.Cu at (106.1, 80.9)
- added R5: 22kR, Resistor_SMD:R_0402_1005Metric, F.Cu at (106.1, 109.9)
- added R6: 22kR, Resistor_SMD:R_0402_1005Metric, F.Cu at (88.7, 75.3)
- added R6: 22kR, Resistor_SMD:R_0402_1005Metric, F.Cu at (88.7, 104.3)
- added REF**: Perforation_0.4mm, Perforation:Perforation_0.4mm, F.Cu at (87.3, 66.9)
- added REF**: Perforation_0.4mm, Perforation:Perforation_0.4mm, F.Cu at (87.3, 97.9)
- added REF**: Perforation_0.4mm, Perforation:Perforation_0.4mm, F.Cu at (108.1, 98.8)
- added REF**: Perforation_0.4mm, Perforation:Perforation_0.4mm, F.Cu at (61.9, 71.8)
- added REF**: Perforation_0.4mm, Perforation:Perforation_0.4mm, F.Cu at (61.9, 100.8)
- added REF**: Perforation_0.4mm, Perforation:Perforation_0.4mm, F.Cu at (108.1, 83.8)
- added REF**: Perforation_0.4mm, Perforation:Perforation_0.4mm, F.Cu at (108.1, 112.8)
- added REF**: Perforation_0.4mm, Perforation:Perforation_0.4mm, F.Cu at (108.1, 84.8)
- added REF**: Perforation_0.4mm, Perforation:Perforation_0.4mm, F.Cu at (108.1, 113.8)
- added REF**: Perforation_0.4mm, Perforation:Perforation_0.4mm, F.Cu at (108.1, 82.8)
- added REF**: Perforation_0.4mm, Perforation:Perforation_0.4mm, F.Cu at (108.1, 111.8)
- added REF**: Perforation_0.4mm, Perforation:Perforation_0.4mm, F.Cu at (108.1, 79.8)
- added REF**: Perforation_0.4mm, Perforation:Perforation_0.4mm, F.Cu at (87.3, 67.9)
- added REF**: Perforation_0.4mm, Perforation:Perforation_0.4mm, F.Cu at (108.1, 108.8)
- added REF**: Perforation_0.4mm, Perforation:Perforation_0.4mm, F.Cu at (61.9, 73.8)
- added REF**: Perforation_0.4mm, Perforation:Perforation_0.4mm, F.Cu at (61.9, 102.8)
- added REF**: Perforation_0.4mm, Perforation:Perforation_0.4mm, F.Cu at (87.3, 96.9)
- added REF**: Perforation_0.4mm, Perforation:Perforation_0.4mm, F.Cu at (82.7, 71.9)
- added REF**: Perforation_0.4mm, Perforation:Perforation_0.4mm, F.Cu at (82.7, 100.9)
- added REF**: Perforation_0.4mm, Perforation:Perforation_0.4mm, F.Cu at (108.1, 77.8)
- added REF**: Perforation_0.4mm, Perforation:Perforation_0.4mm, F.Cu at (108.1, 106.8)
- added REF**: Perforation_0.4mm, Perforation:Perforation_0.4mm, F.Cu at (108.1, 70.8)
- added REF**: Perforation_0.4mm, Perforation:Perforation_0.4mm, F.Cu at (108.1, 99.8)
- added REF**: Perforation_0.4mm, Perforation:Perforation_0.4mm, F.Cu at (82.7, 67.9)
- added REF**: Perforation_0.4mm, Perforation:Perforation_0.4mm, F.Cu at (87.3, 95.9)
- added REF**: Perforation_0.4mm, Perforation:Perforation_0.4mm, F.Cu at (82.7, 96.9)
- added REF**: Perforation_0.4mm, Perforation:Perforation_0.4mm, F.Cu at (108.1, 71.8)
- added REF**: Perforation_0.4mm, Perforation:Perforation_0.4mm, F.Cu at (108.1, 100.8)
- added REF**: Perforation_0.4mm, Perforation:Perforation_0.4mm, F.Cu at (108.1, 72.8)
- added REF**: Perforation_0.4mm, Perforation:Perforation_0.4mm, F.Cu at (108.1, 101.8)
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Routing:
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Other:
- outline, holes or cut-outs redrawn
